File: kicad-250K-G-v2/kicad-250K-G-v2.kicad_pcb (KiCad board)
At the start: 2 copper layers, 28 parts, among them P1 In, P2 Out, P3 Power, U1 TL072

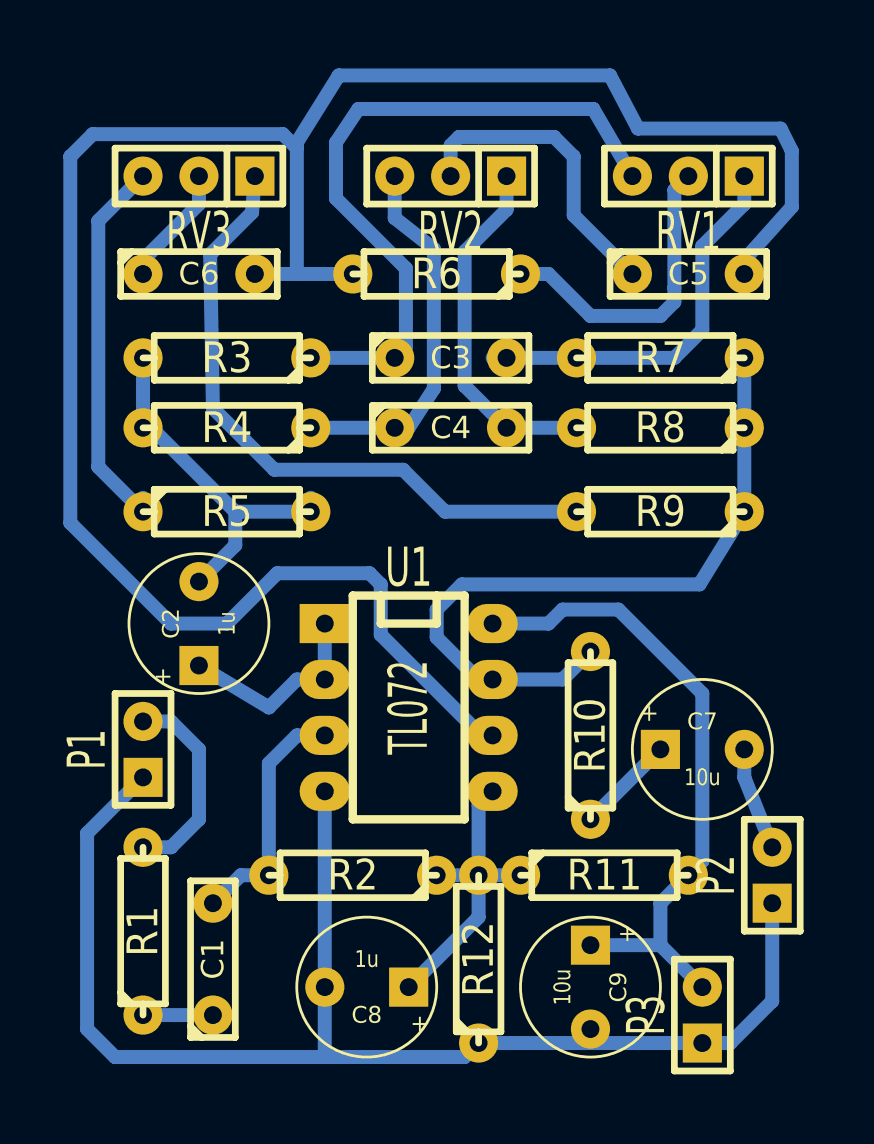
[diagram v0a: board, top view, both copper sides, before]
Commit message: routing corrections
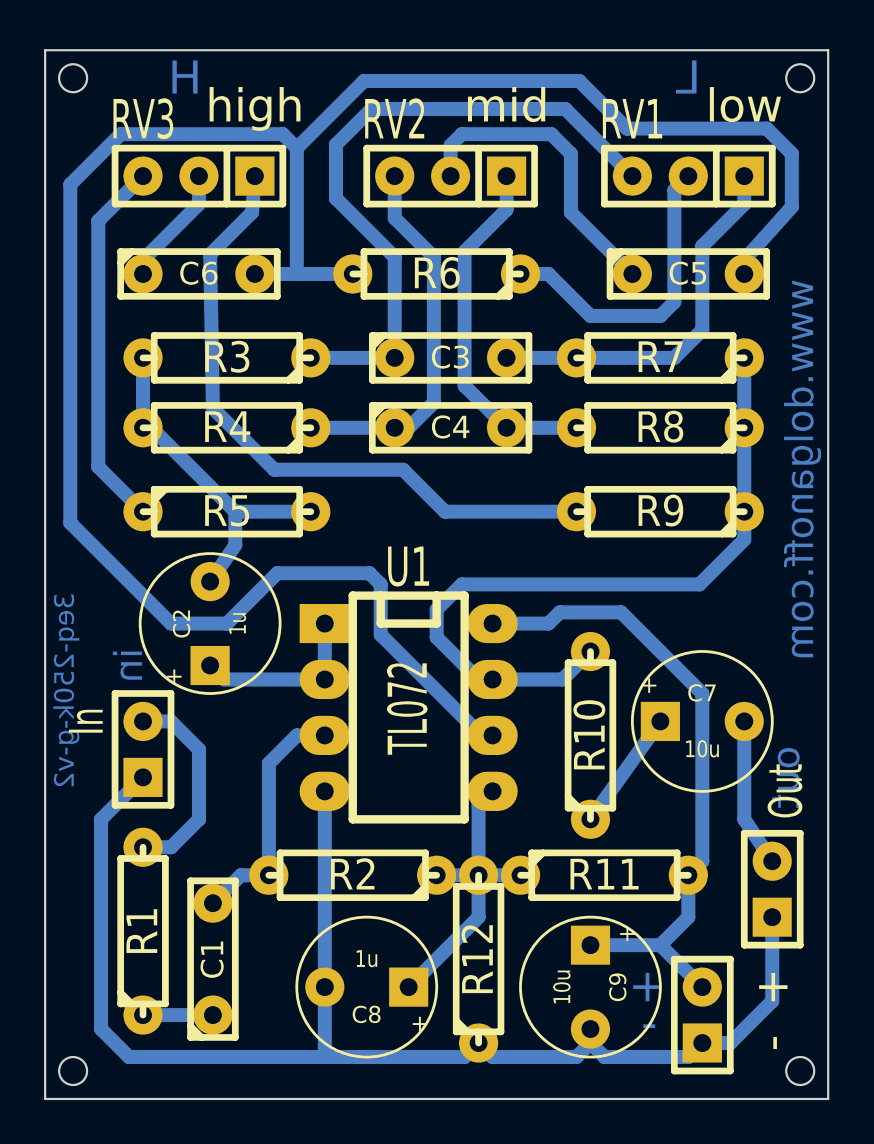
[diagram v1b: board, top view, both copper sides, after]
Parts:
- moved C7 1.27 mm to (142.2, 106.7)
- moved P2 0.63 mm to (145.4, 114.3)
- moved C2 0.51 mm to (119.9, 102.2)
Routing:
- net Net-(C5-Pad2): track 97.7 -> 95.5 mm
- net Net-(C7-Pad2): track 4.69 -> 6.73 mm
- net Net-(C2-Pad1): track 9.31 -> 8.01 mm
- net Net-(C3-Pad1): track 31.1 -> 30.0 mm
- net Net-(C7-Pad1): track 4.49 -> 5.46 mm
- net Net-(C2-Pad2): track 16.9 -> 15.9 mm
- net Net-(R5-Pad1): track 17.6 -> 16.9 mm
- net Net-(C3-Pad2): track 17.8 -> 17.2 mm
- net Net-(C5-Pad1): track 14.6 -> 14.1 mm
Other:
- board outline added: 35.6 x 47.6 mm
- board text added: "+"
- board text added: "-"
- board text added: "3eq-250k-g-v2"
- board text added: "H"
- board text added: "L"
- board text added: "high"
- board text added: "in"
- board text added: "low"
- board text added: "mid"
- board text added: "out"
- board text added: "www.dolganoff.com"
